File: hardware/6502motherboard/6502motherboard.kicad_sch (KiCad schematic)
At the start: 25 parts, among them J1 AUX 5VDC, J2 POWER 5V, J3 GND, SW1 POWER, SW2 SW_Push, T1 DS-1813, U3 74HCT273

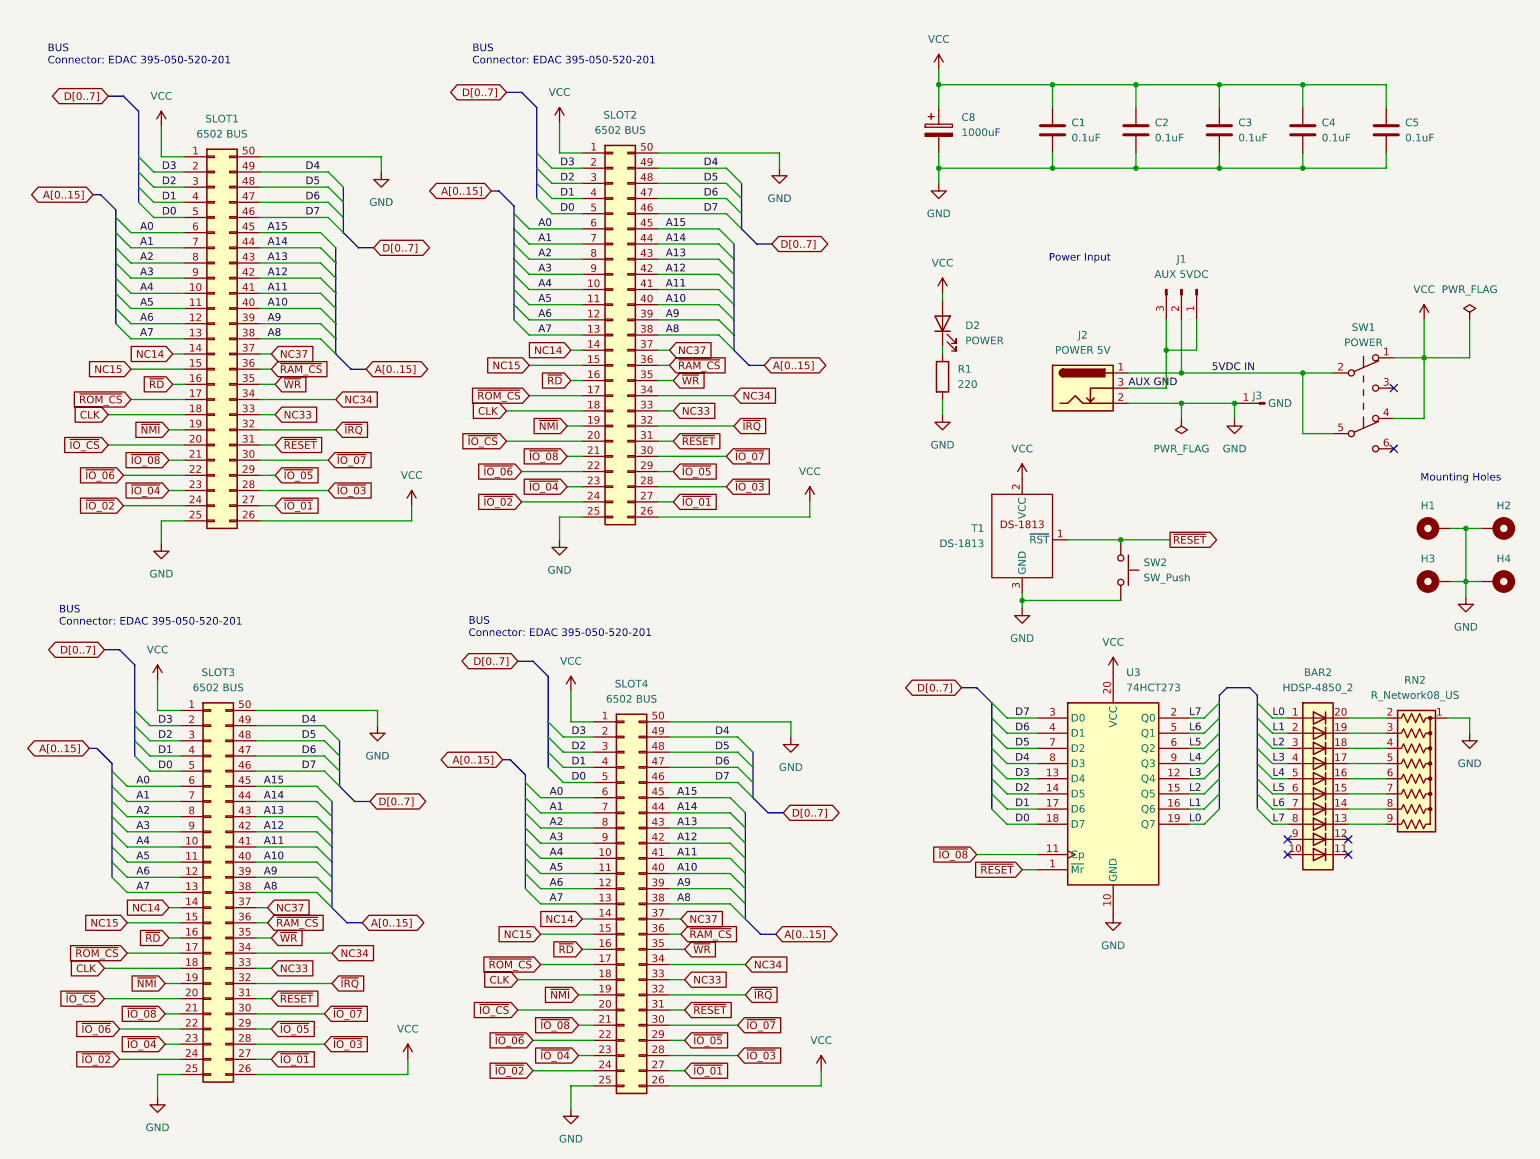
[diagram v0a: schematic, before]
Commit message: v1.6 Motherboard Complete
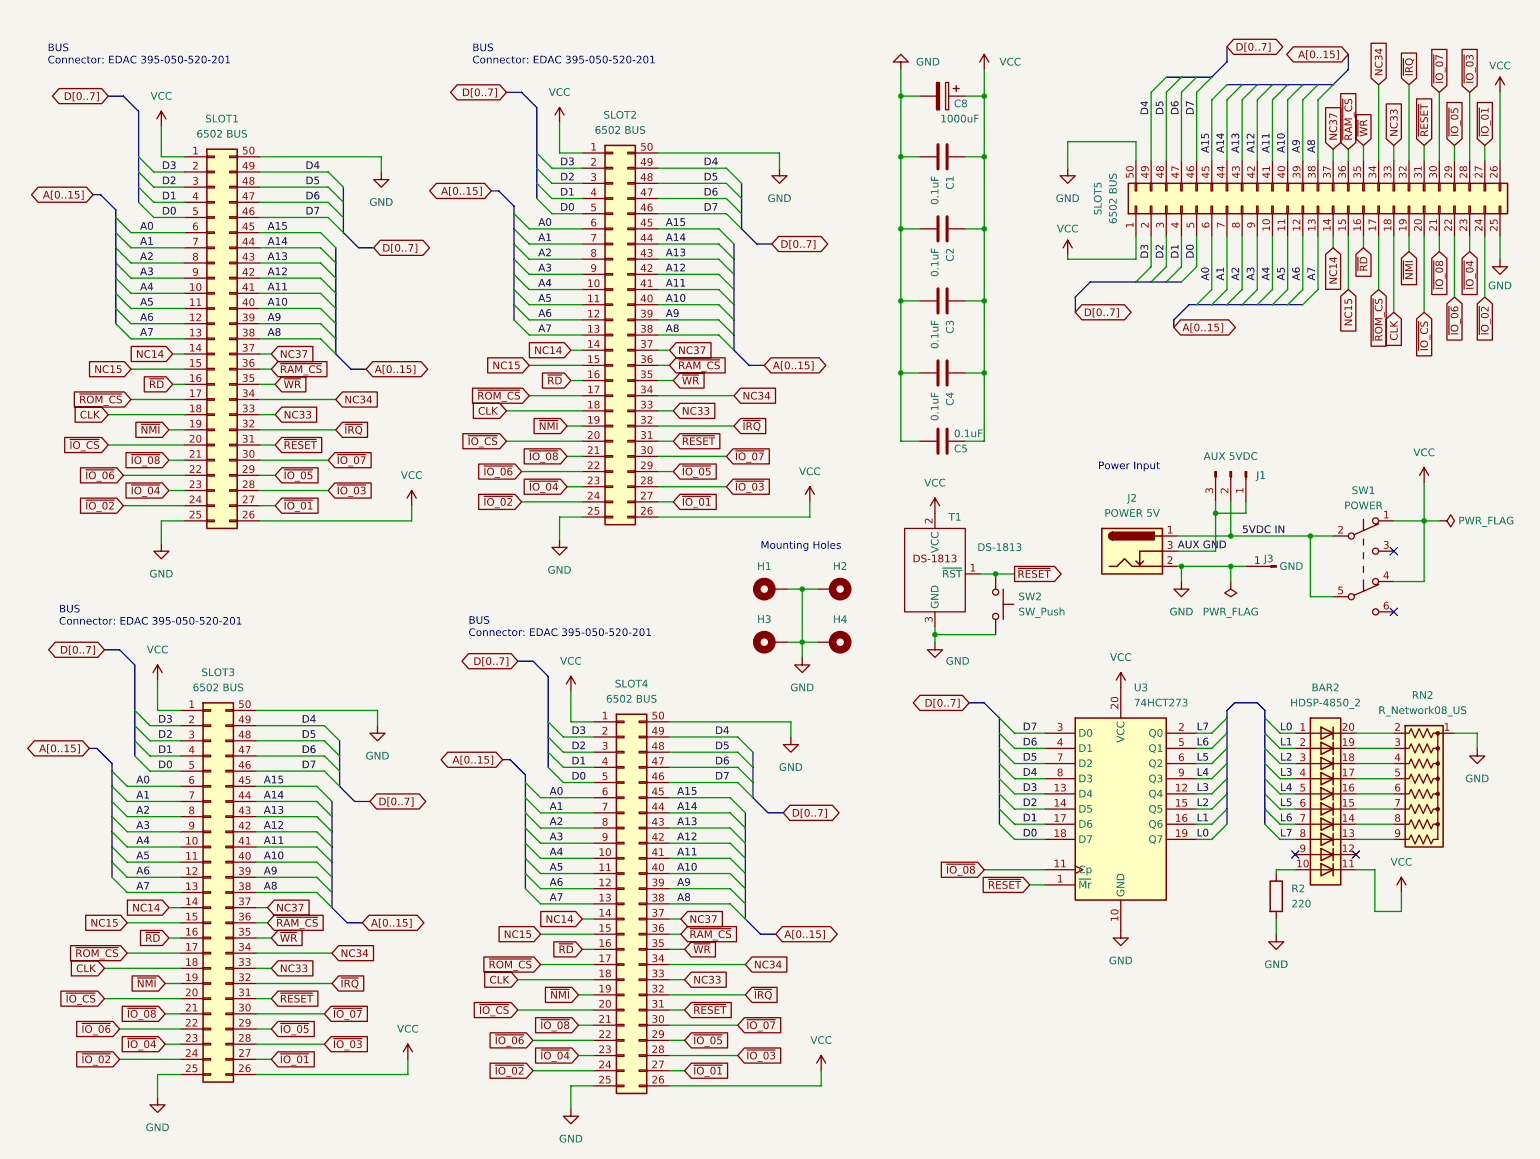
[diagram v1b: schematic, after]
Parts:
- removed D2: POWER, LED_THT:LED_D3.0mm, symbol Device:LED
- removed R1: 220, Resistor_THT:R_Axial_DIN0204_L3.6mm_D1.6mm_P7.62mm_Horizontal, symbol Device:R
- added R2: 220, Resistor_THT:R_Axial_DIN0204_L3.6mm_D1.6mm_P7.62mm_Horizontal, symbol Device:R
- added SLOT5: 6502 BUS, Connector_PinHeader_2.54mm:PinHeader_2x25_P2.54mm_Vertical_Counter_Clockwise, symbol Connector_Generic:Conn_02x25_Counter_Clockwise
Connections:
- net A0: now also SLOT5.6 (Pin_6)
- net A1: now also SLOT5.7 (Pin_7)
- net A10: now also SLOT5.40 (Pin_40)
- net A11: now also SLOT5.41 (Pin_41)
- net A12: now also SLOT5.42 (Pin_42)
- net A13: now also SLOT5.43 (Pin_43)
- net A14: now also SLOT5.44 (Pin_44)
- net A15: now also SLOT5.45 (Pin_45)
- net A2: now also SLOT5.8 (Pin_8)
- net A3: now also SLOT5.9 (Pin_9)
- net A4: now also SLOT5.10 (Pin_10)
- net A5: now also SLOT5.11 (Pin_11)
- net A6: now also SLOT5.12 (Pin_12)
- net A7: now also SLOT5.13 (Pin_13)
- net A8: now also SLOT5.38 (Pin_38)
- net A9: now also SLOT5.39 (Pin_39)
- net CLK: now also SLOT5.18 (Pin_18)
- net D0: now also SLOT5.5 (Pin_5)
- net D1: now also SLOT5.4 (Pin_4)
- net D2: now also SLOT5.3 (Pin_3)
- net D3: now also SLOT5.2 (Pin_2)
- net D4: now also SLOT5.49 (Pin_49)
- net D5: now also SLOT5.48 (Pin_48)
- net D6: now also SLOT5.47 (Pin_47)
- net D7: now also SLOT5.46 (Pin_46)
- net GND: now also R2.2, SLOT5.25 (Pin_25), SLOT5.50 (Pin_50)
- net NC14: now also SLOT5.14 (Pin_14)
- net NC15: now also SLOT5.15 (Pin_15)
- net NC33: now also SLOT5.33 (Pin_33)
- net NC34: now also SLOT5.34 (Pin_34)
- net NC37: now also SLOT5.37 (Pin_37)
- net VCC: now also BAR2.11 (K), SLOT5.1 (Pin_1), SLOT5.26 (Pin_26)
- net ~{IO_01}: now also SLOT5.27 (Pin_27)
- net ~{IO_02}: now also SLOT5.24 (Pin_24)
- net ~{IO_03}: now also SLOT5.28 (Pin_28)
- net ~{IO_04}: now also SLOT5.23 (Pin_23)
- net ~{IO_05}: now also SLOT5.29 (Pin_29)
- net ~{IO_06}: now also SLOT5.22 (Pin_22)
- net ~{IO_07}: now also SLOT5.30 (Pin_30)
- net ~{IO_08}: now also SLOT5.21 (Pin_21)
- net ~{IO_CS}: now also SLOT5.20 (Pin_20)
- net ~{IRQ}: now also SLOT5.32 (Pin_32)
- net ~{NMI}: now also SLOT5.19 (Pin_19)
- net ~{RAM_CS}: now also SLOT5.36 (Pin_36)
- net ~{RD}: now also SLOT5.16 (Pin_16)
- net ~{RESET}: now also SLOT5.31 (Pin_31)
- net ~{ROM_CS}: now also SLOT5.17 (Pin_17)
- net ~{WR}: now also SLOT5.35 (Pin_35)
- net at BAR2.10 (A): now also R2.1
- no-connect marks 6 -> 4
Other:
- moved on the sheet: BAR2, C1, C2, C3, C4, C5, C8, H1, H2, H3, H4, J1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
